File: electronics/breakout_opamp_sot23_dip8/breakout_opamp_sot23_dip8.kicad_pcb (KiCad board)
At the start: 2 copper layers, 11.4 x 11.4 mm, 6 parts, among them J1 Conn_01x04, J2 Conn_01x04

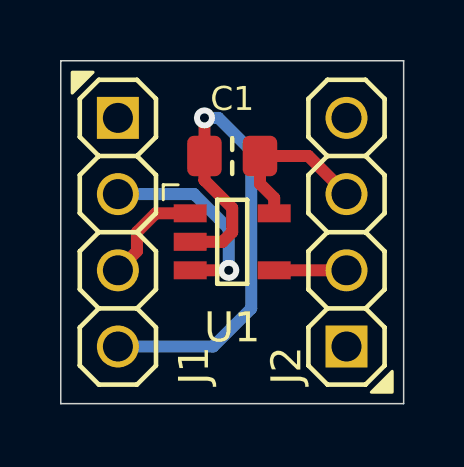
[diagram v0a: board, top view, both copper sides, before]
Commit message: preparation for production
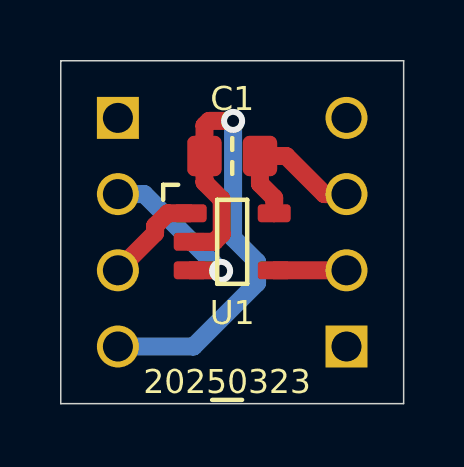
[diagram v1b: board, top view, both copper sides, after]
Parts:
- removed N2: OHWLOGO, Symbol:OSHW-Symbol_6.7x6mm_SilkScreen
- J1, J2: moved to B.Cu
- N1: value 20240915 -> 20250323; moved to F.Cu
- moved N1 10.1 mm to (128.1, 59.6), turned to 0 degrees
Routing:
- net /-IN: track 6.84 -> 5.54 mm
- net /V-: track 18.0 -> 17.3 mm
